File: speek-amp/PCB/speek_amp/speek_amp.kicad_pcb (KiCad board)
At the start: 2 copper layers, 120 x 80 mm, 102 parts, among them U1 TPA3116D2DAD_C2865736, U10 TPA3116D2DAD_C2865736, U11 R_Tweeter, U12 R_Woofer, U13 10uH, U14 10uH, U15 L_Tweeter, U16 L_Woofer, U17 L_Sub, U18 J1, U2 10uH, U3 10uH, U4 XT60, U5 10uH, U6 10uH, U7 PDMTAT068125-151MLU, U8 PDMTAT068125-151MLU, U9 50PX4700MEFC18X40

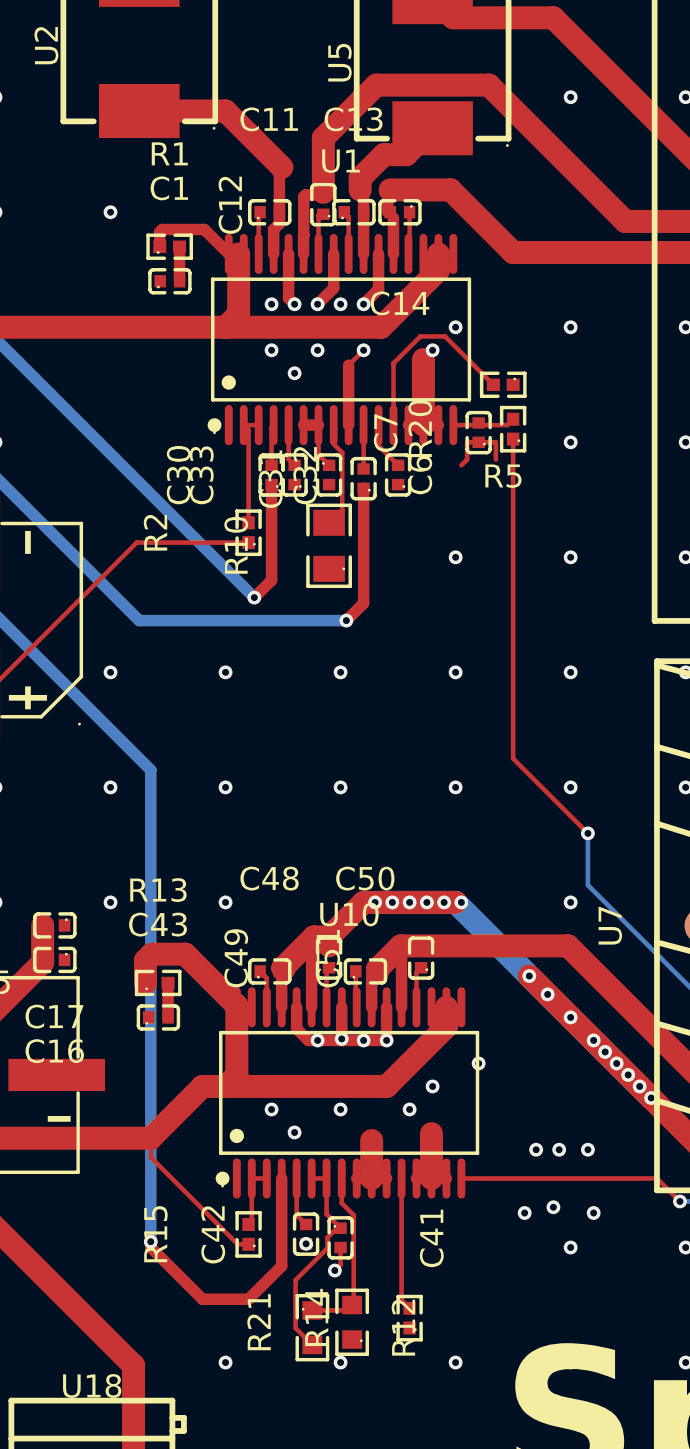
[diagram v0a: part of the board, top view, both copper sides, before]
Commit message: wowoowww
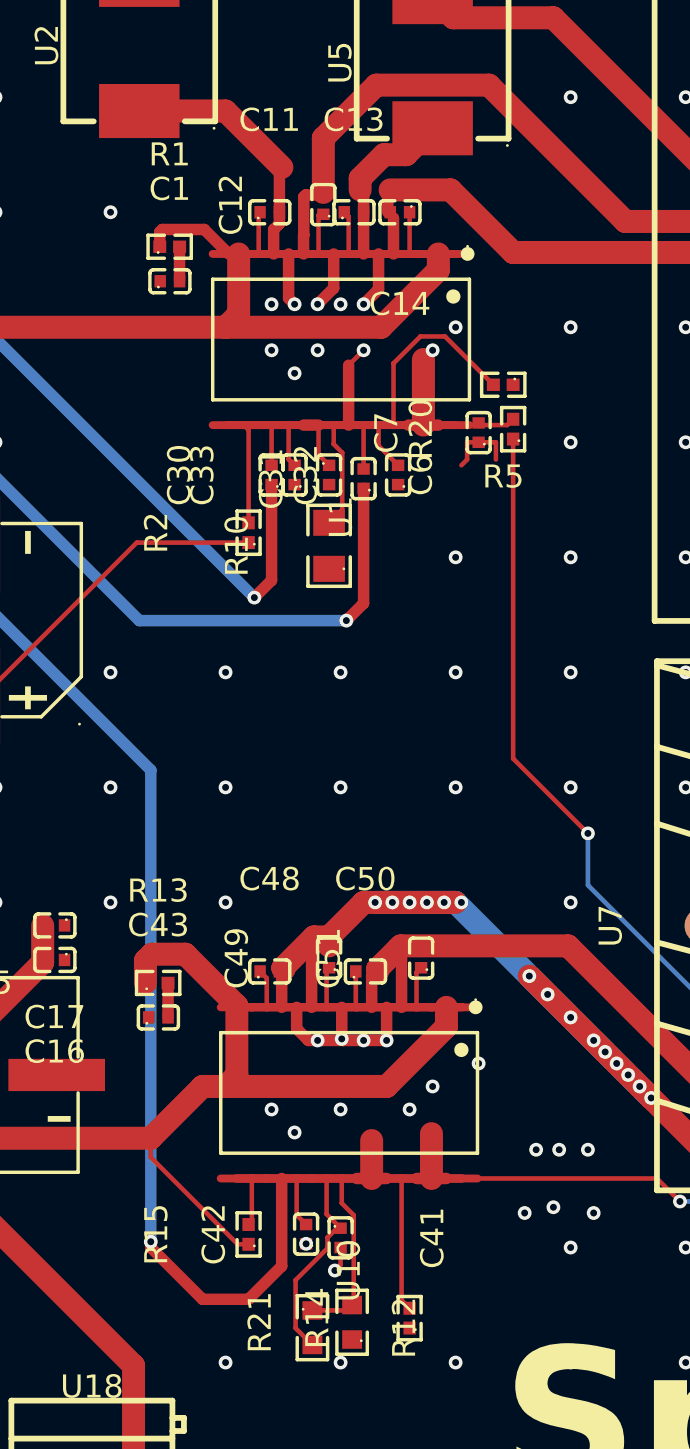
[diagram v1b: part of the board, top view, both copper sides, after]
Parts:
- turned U1 to 90 degrees
- turned U10 to 90 degrees

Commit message: redoc
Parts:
- turned U1 to -90 degrees
- turned U10 to -90 degrees
